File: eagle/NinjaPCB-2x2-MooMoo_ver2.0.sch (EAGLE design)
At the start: 69 parts, among them IC1 ANALOGSW_AD_SOT23-6, IC2 NAU7802, Q1 IRLB3813PBF, Q2 CJ2302, Q3 CJ2302, Q4 S9013, Q5 S9013, Q6 S9013, T1 TPTP20R, T2 TPTP20R, T3 TPTP20R, T4 TPTP20R, T5 TPTP20R, T6 TPTP20R, T7 TPTP20R

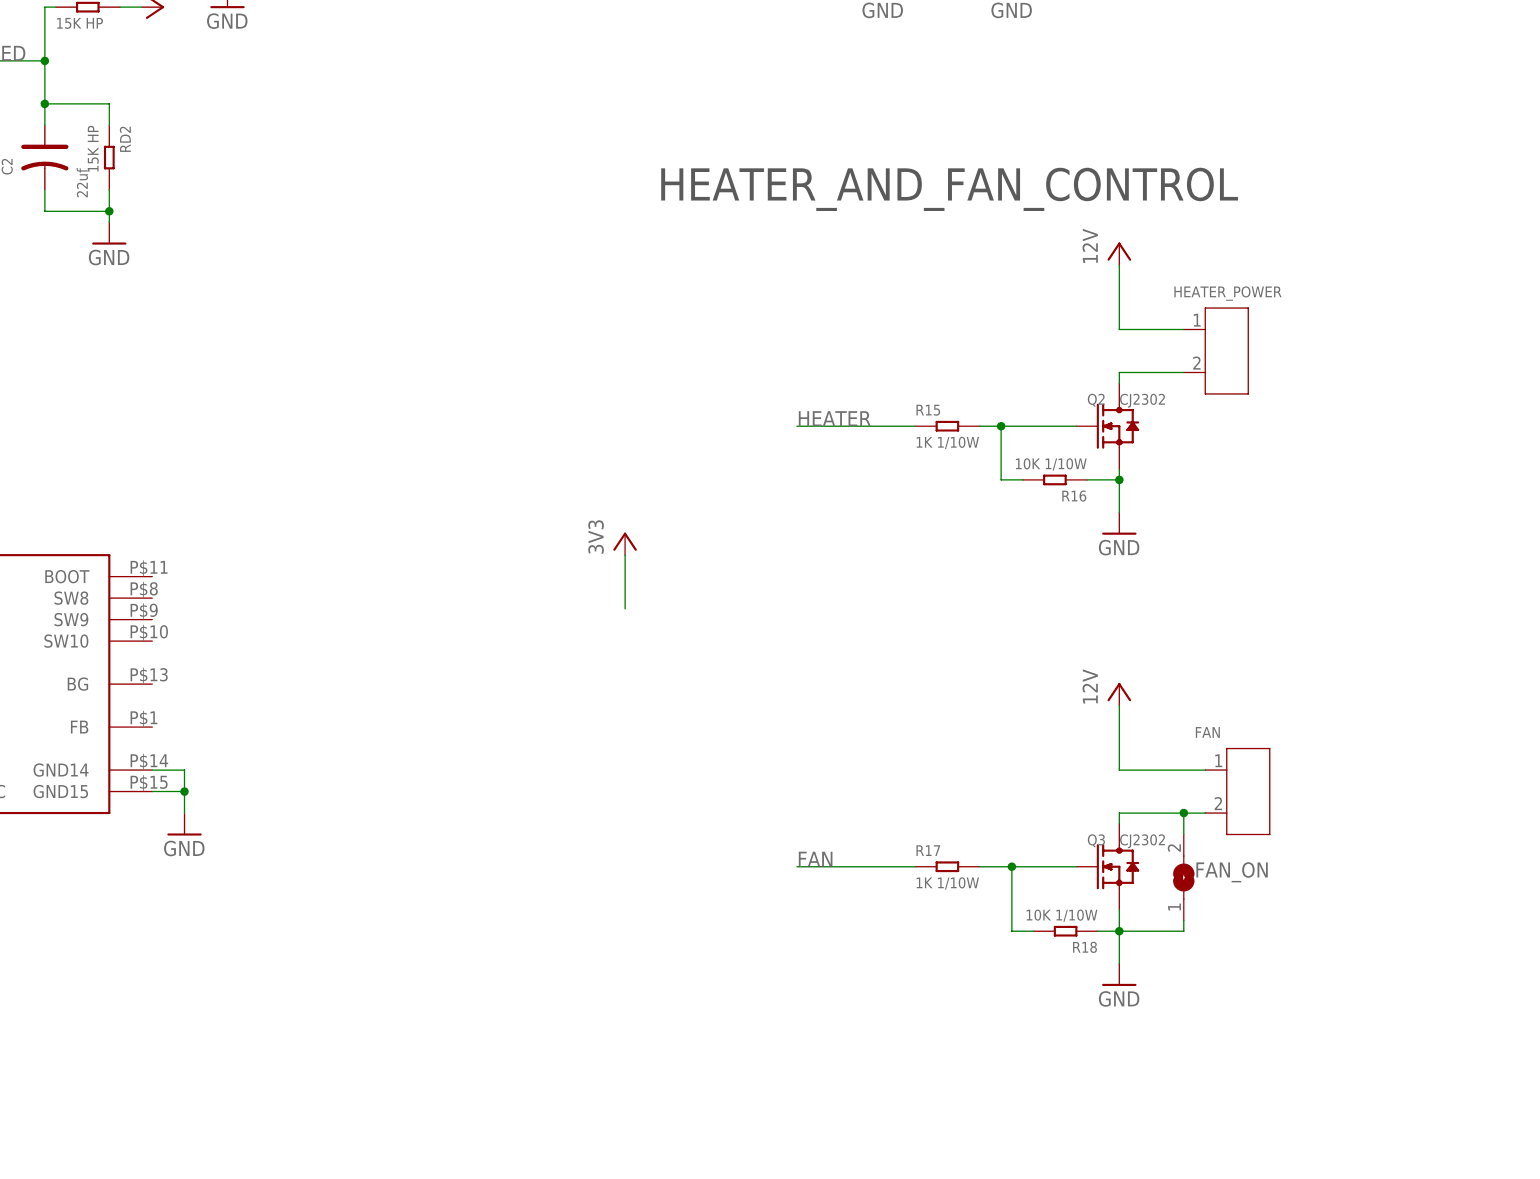
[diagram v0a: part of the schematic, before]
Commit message: ordered
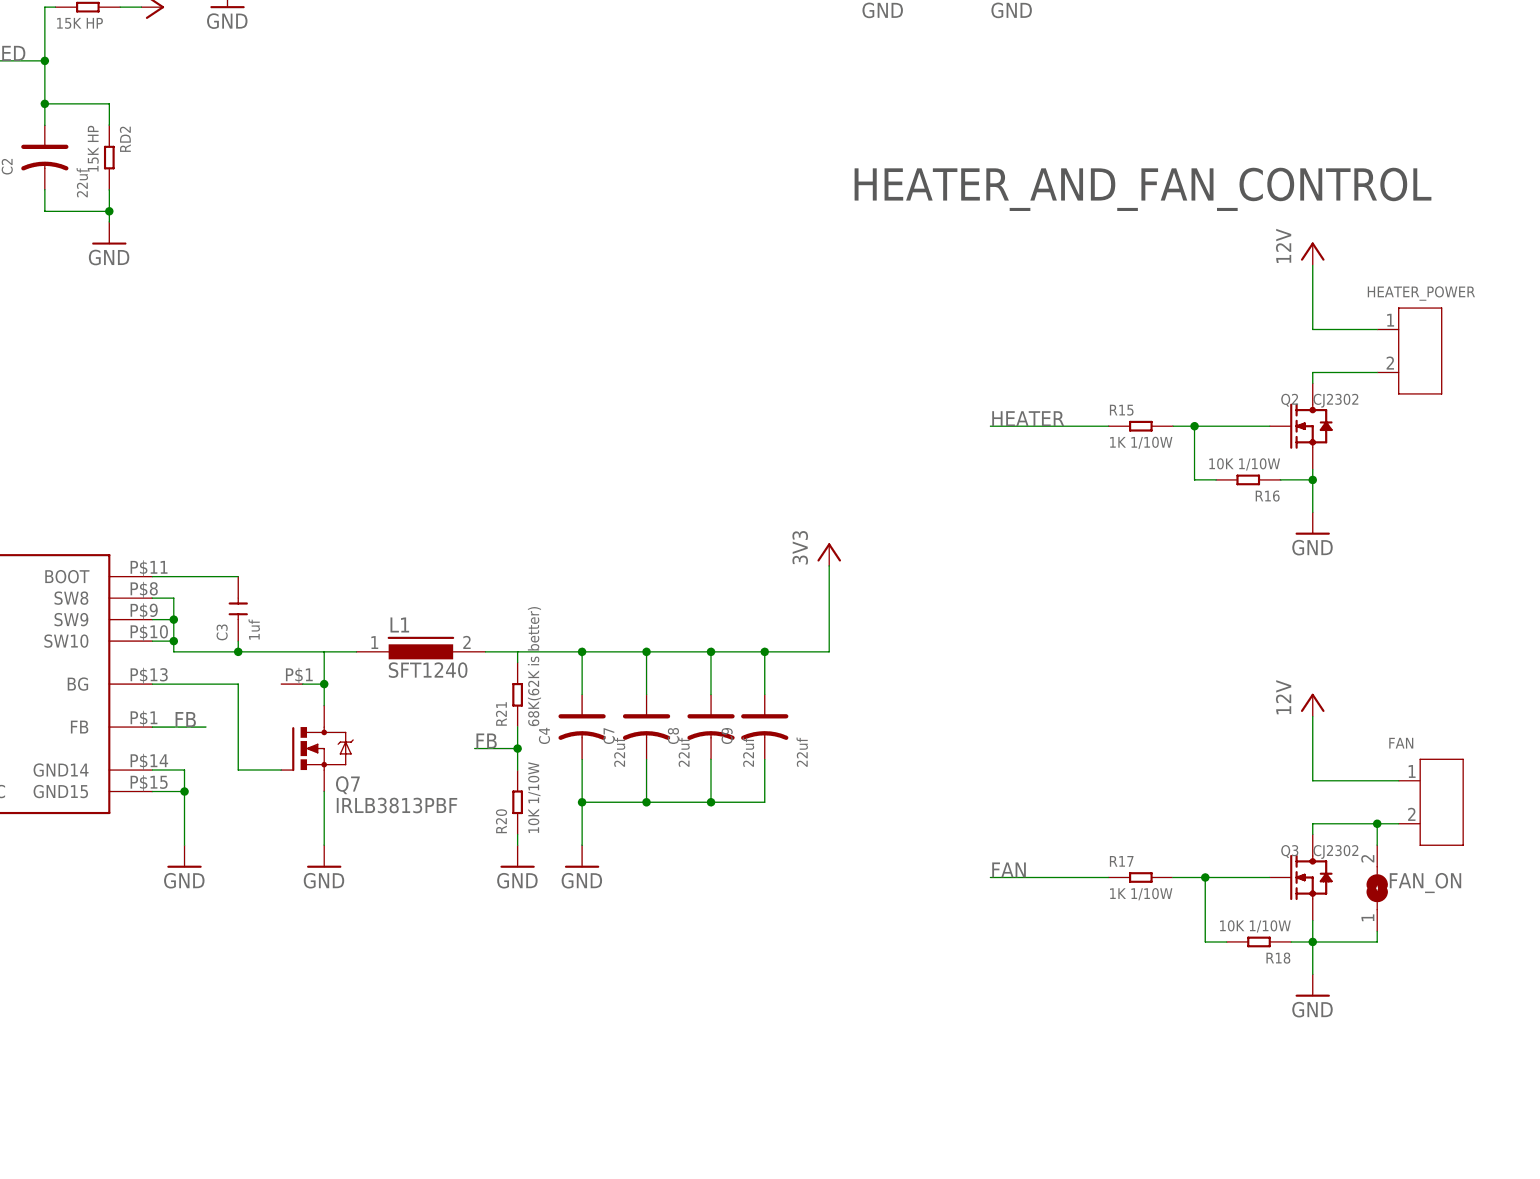
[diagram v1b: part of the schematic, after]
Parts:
- added C3: 1uf, Seeed-Capacitor:CERAMIC-1UF-25V-10%-X7R(0603)
- added C4, C7, C8, C9: 22uf, Seeed-Capacitor:TANTALUM-SMD-22UF-16V(AVX-B)
- added HEATSINK1: HEAT111PB015, PCR-Connector:HEAT111PB015
- added L1: SFT1240, inductors:SFT1240
- added Q7: IRLB3813PBF, transistor-power:IRF520
- added R20: 10K 1/10W, Seeed-Resistor:SMD-RES-10K-5%-1/10W(0603)
- added R21: 68K(62K is better), Seeed-Resistor:SMD-RES-30K-5%-1/10W(0603)
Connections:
- new net FB: R20.2, R21.1, REG.FB
- new net N$13: C3.2, REG.BOOT
- new net N$14: C3.1, HEATSINK1.P$1, L1.1, Q7.D, REG.SW10, REG.SW8, REG.SW9
- new net N$15: Q7.G, REG.BG
- net 3V3: now also C4.+, C7.+, C8.+, C9.+, L1.2, R21.2
- net GND: now also C4.-, C7.-, C8.-, C9.-, Q7.S, R20.1
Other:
- moved on the sheet: FAN, FAN_ON, HEATER_POWER, Q2, Q3, R15, R16, R17, R18
